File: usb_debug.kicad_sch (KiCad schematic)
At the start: 12 parts, among them J5 USB_C_Receptacle_USB2.0, U1 MIMXRT1052CVJ5B, U7 PRTR5V0U2X, U8 XC6206P332PR-G

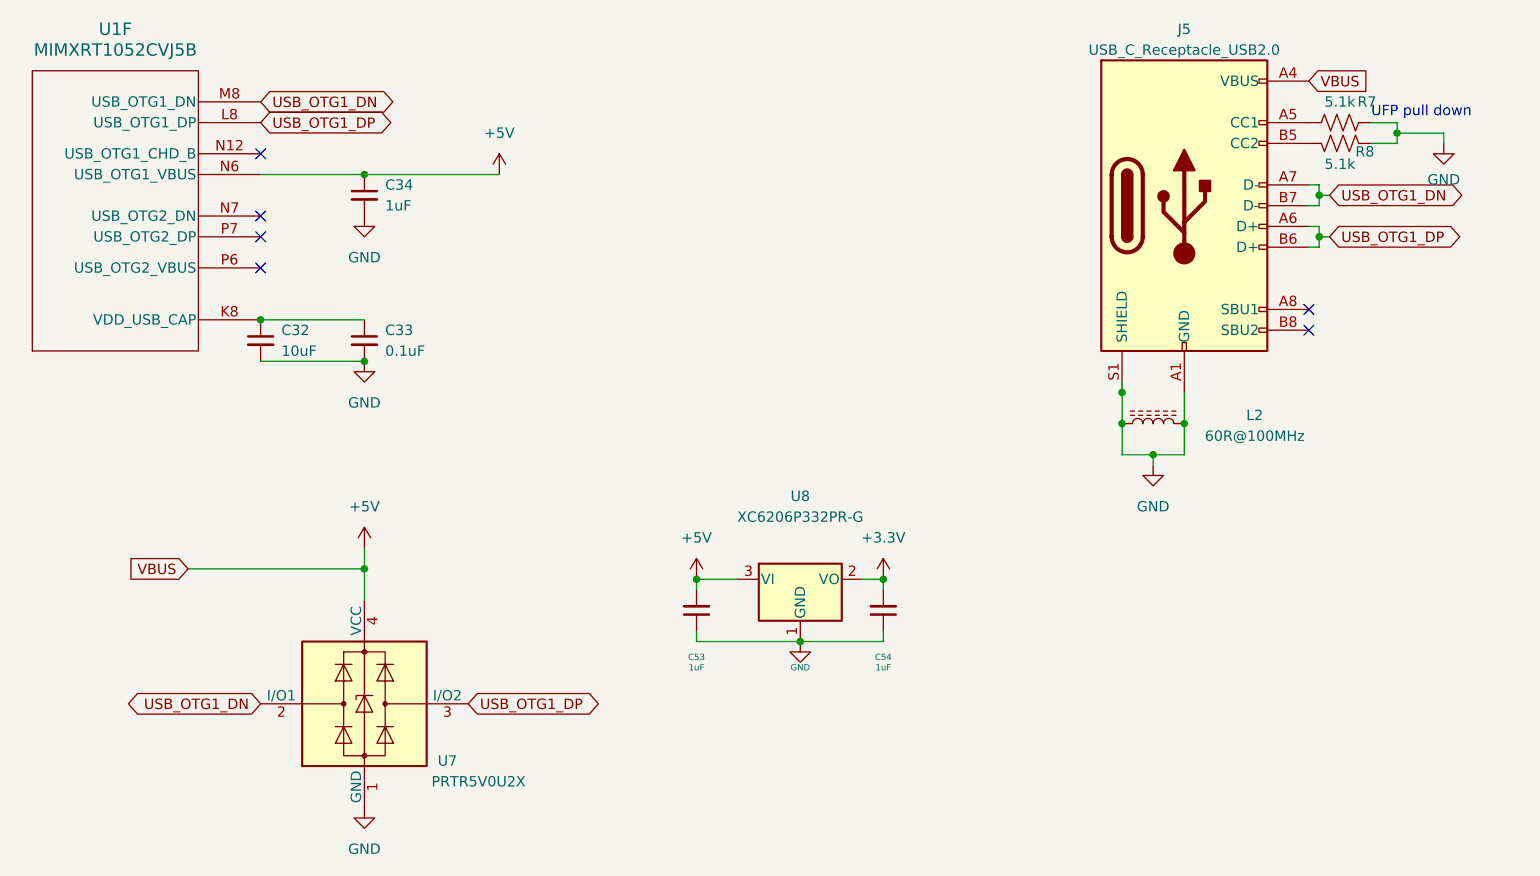
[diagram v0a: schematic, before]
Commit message: save before sdram redesign
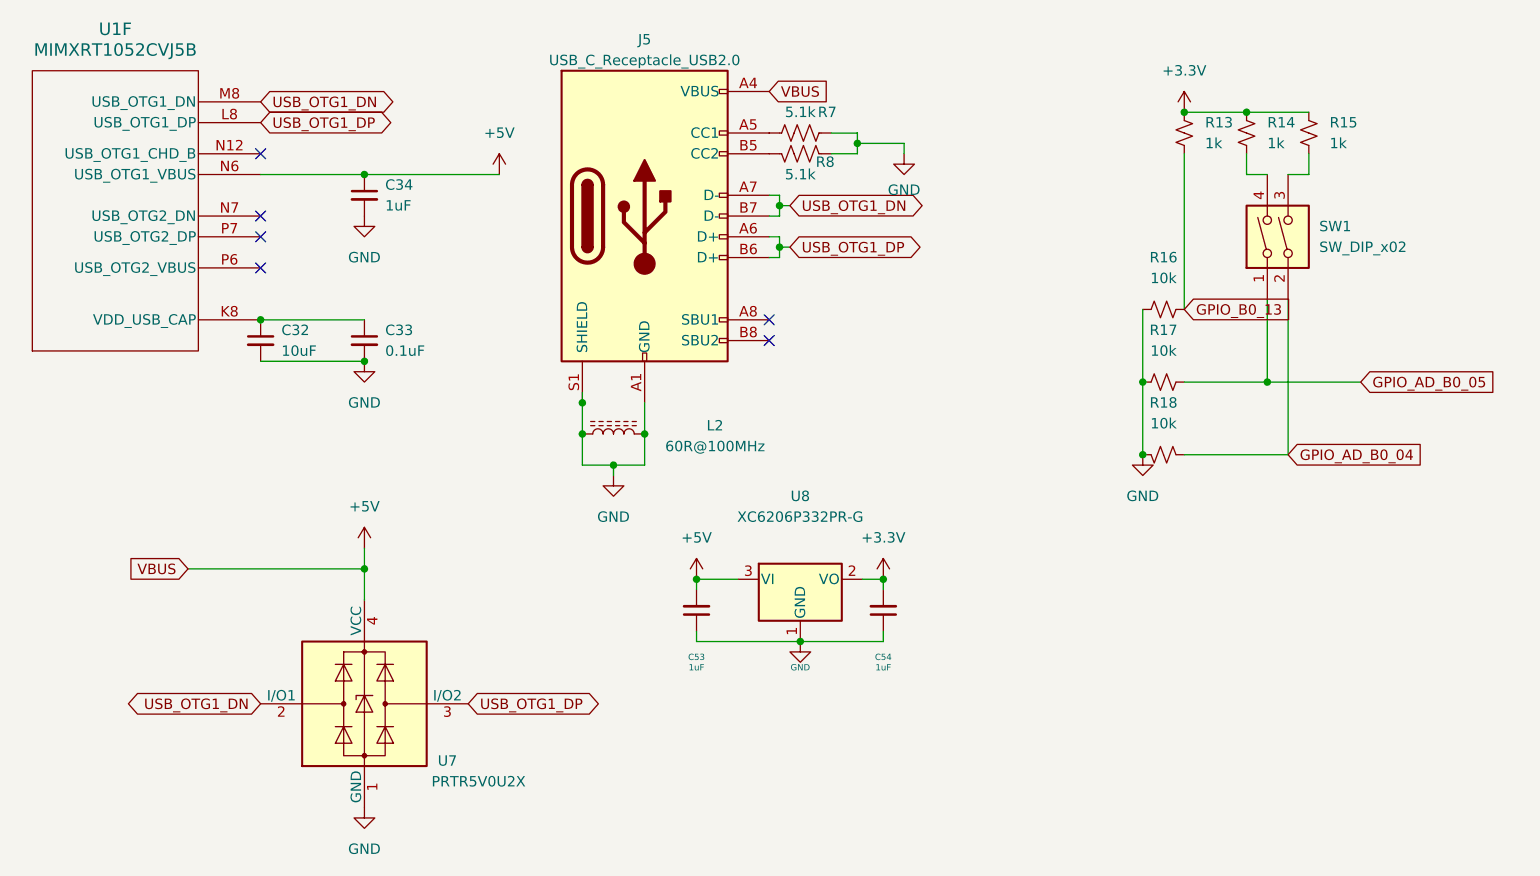
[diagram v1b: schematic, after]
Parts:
- added R13, R14, R15: 1k, Resistor_SMD:R_0402_1005Metric, symbol Device:R_Small_US
- added R16, R17, R18: 10k, Resistor_SMD:R_0402_1005Metric, symbol Device:R_Small_US
- added SW1: SW_DIP_x02, Button_Switch_SMD:SW_DIP_SPSTx02_Slide_6.7x6.64mm_W6.73mm_P2.54mm_LowProfile_JPin, symbol Switch:SW_DIP_x02
- C32, C33, C34, C53, C54: footprint Capacitor_SMD:C_0402_1005Metric -> Capacitor_SMD:C_0201_0603Metric
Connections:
- net +3.3V: now also R13.1, R14.1, R15.1
- net GND: now also R16.1, R17.1, R18.2
- new net: R15.2, SW1.3
- new net: R14.2, SW1.4
- new net GPIO_AD_B0_04: R18.1, SW1.2
- new net GPIO_AD_B0_05: R17.2, SW1.1
- new net GPIO_B0_13: R13.2, R16.2
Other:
- note removed: "UFP pull down"
- moved on the sheet: J5, L2, R7, R8
